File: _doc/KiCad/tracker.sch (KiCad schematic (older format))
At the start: 16 parts

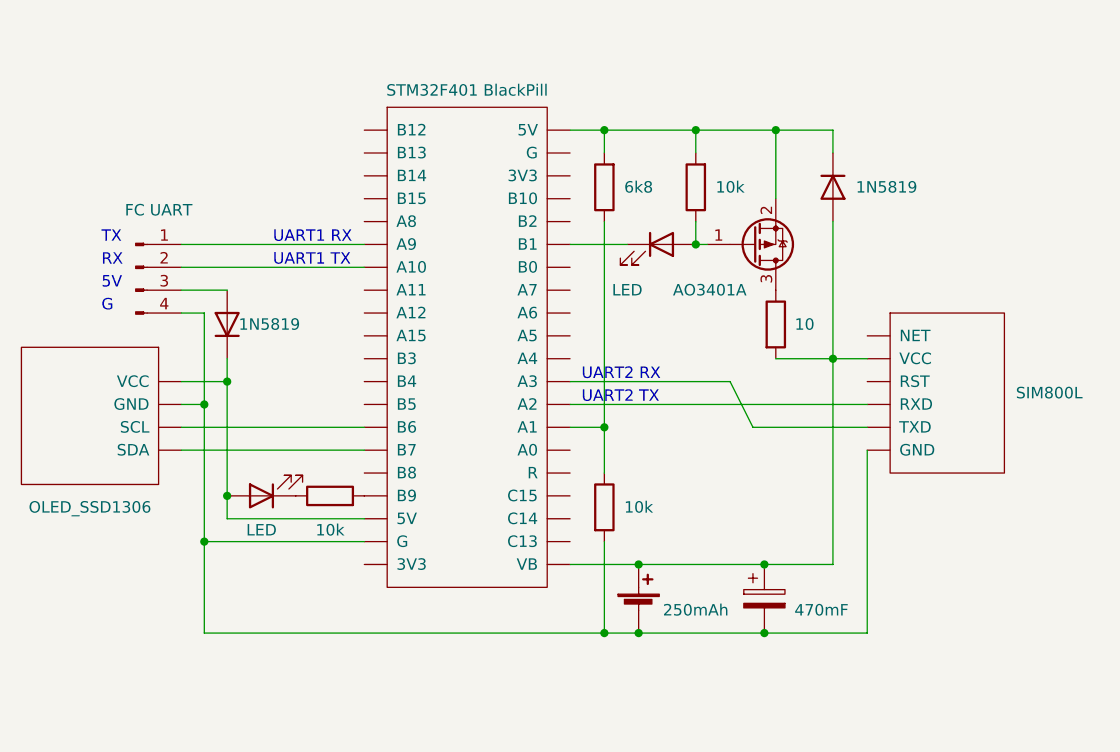
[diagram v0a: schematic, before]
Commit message: Doc: schematic
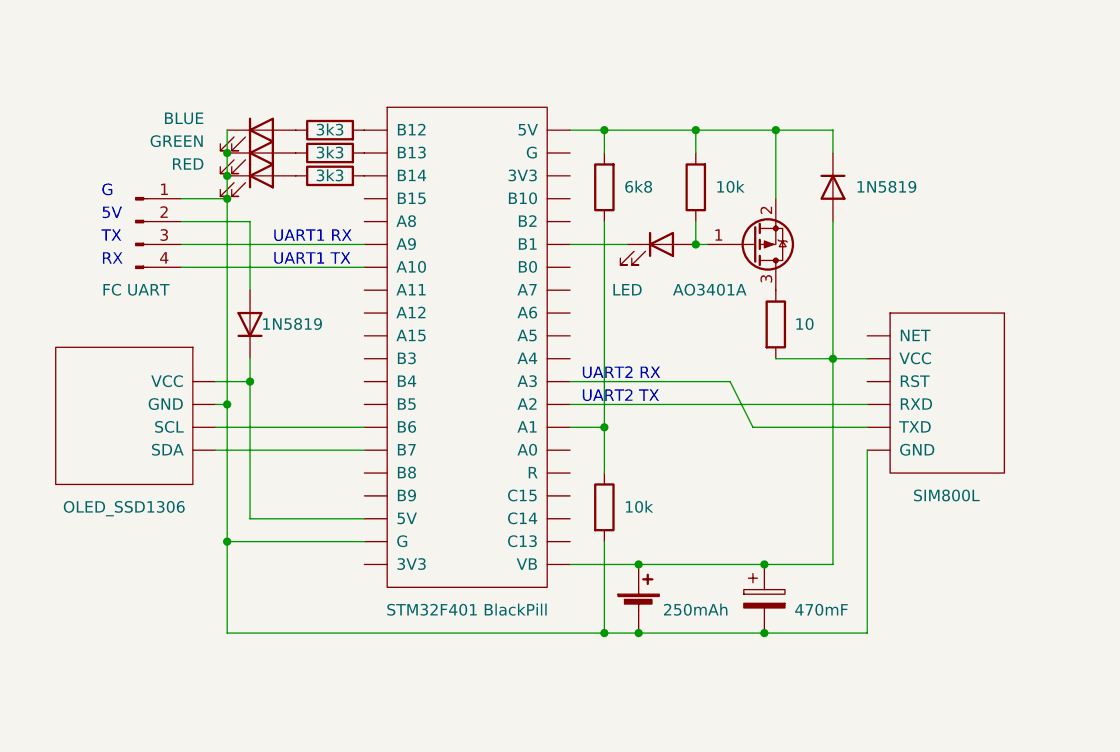
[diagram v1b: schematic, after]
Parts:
- added D?: GREEN, symbol Device:LED
- added D?: RED, symbol Device:LED
- added R? (x2): 3k3, symbol Device:R
- D?: value LED -> BLUE
- R?: value 10k -> 3k3
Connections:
- net at U?.~ (VB): now also R?.2
- net at U?.~ (VCC): no longer U?.~ (VB)
- net at U?.~ (VB), U?.~ (VCC): now also D?.1 (K)
- net at J?.1 (Pin_1), U?.~ (VB): now also BT?.2 (-), C?.2, D?.1 (K), R?.2, U?.~ (VCC), U?.~ (VCC), D?.1 (K), D?.1 (K)
- net at J?.2 (Pin_2): now also D?.2 (A); no longer U?.~ (VB)
- net at J?.3 (Pin_3): now also U?.~ (VB); no longer D?.2 (A)
- net at R?.1: now also D?.2 (A); no longer D?.1 (K)
- new net: U?.~ (VB), U?.~ (VCC) (x4)
- new net: J?.4 (Pin_4), U?.~ (VB)
- new net: R?.2, U?.~ (VB) (x2)
- new net: D?.2 (A), R?.1 (x2)
- now unconnected: U?.~ (VCC), U?.~ (VCC)
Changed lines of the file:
@@
 P 7100 3750
 F 0 "U?" H 7378 3796 50  0001 L CNN
-F 1 "SIM800L" H 7400 3750 50  0000 L CNN
+F 1 "SIM800L" H 6950 3300 50  0000 L CNN
 F 2 "" H 7100 4150 50  0001 C CNN
 F 3 "" H 7100 4150 50  0001 C CNN
@@
 $EndComp
 Wire Wire Line
-	3850 4400 4550 4400
-Wire Wire Line
-	3950 3700 3950 4200
-Wire Wire Line
-	3950 4300 4550 4300
-Wire Wire Line
-	3850 3800 3850 4400
-Connection ~ 3950 3700
-Wire Wire Line
-	3850 3400 3850 3800
-Connection ~ 3850 3800
-Wire Wire Line
-	3850 4400 3850 4800
-Connection ~ 3850 4400
+	3950 4400 4550 4400
+Wire Wire Line
+	4050 4300 4550 4300
+Wire Wire Line
+	3950 3800 3950 4400
+Connection ~ 4050 3700
+Connection ~ 3950 3800
+Wire Wire Line
+	3950 4400 3950 4800
+Connection ~ 3950 4400
 Wire Wire Line
 	5450 3700 6150 3700
 Wire Wire Line
-	3950 3600 3950 3700
+	4050 3600 4050 3700
 $Comp
 L Device:Battery_Cell BT?
@@
 $EndComp
 Wire Wire Line
-	3850 4800 5600 4800
+	3950 4800 5600 4800
 Connection ~ 5750 4500
 Wire Wire Line
@@
 Text Notes 3400 3200 0    50   ~ 0
 RX
-Text Notes 3400 3300 0    50   ~ 0
+Text Notes 3400 3000 0    50   ~ 0
 5V
-Text Notes 3400 3400 0    50   ~ 0
-G
 Connection ~ 6350 2600
 Wire Wire Line
@@
 L Device:D D?
 U 1 1 5FC14E46
-P 3950 3450
-F 0 "D?" V 4050 3400 50  0001 R CNN
-F 1 "1N5819" V 3950 3400 50  0000 R CNN
-F 2 "" H 3950 3450 50  0001 C CNN
-F 3 "~" H 3950 3450 50  0001 C CNN
-	1    3950 3450
+P 4050 3450
+F 0 "D?" V 4150 3400 50  0001 R CNN
+F 1 "1N5819" V 4050 3400 50  0000 R CNN
+F 2 "" H 4050 3450 50  0001 C CNN
+F 3 "~" H 4050 3450 50  0001 C CNN
+	1    4050 3450
 	0    -1   -1   0
 $EndComp
@@
 L myLib:OLED_SSD1306 U?
 U 1 1 5FBCCE2D
-P 3350 3850
-F 0 "U?" H 3350 3500 50  0001 C CNN
-F 1 "OLED_SSD1306" H 3350 3450 50  0000 C CNN
-F 2 "" H 3350 4250 50  0001 C CNN
-F 3 "" H 3350 4250 50  0001 C CNN
-	1    3350 3850
-	1    0    0    -1
-$EndComp
-Wire Wire Line
-	3750 3800 3850 3800
-Wire Wire Line
-	3750 3900 4550 3900
-Wire Wire Line
-	4550 4000 3750 4000
-Wire Wire Line
-	3750 3700 3950 3700
-Wire Wire Line
-	3750 3400 3850 3400
-Wire Wire Line
-	3750 3300 3950 3300
+P 3500 3850
+F 0 "U?" H 3500 3500 50  0001 C CNN
+F 1 "OLED_SSD1306" H 3500 3450 50  0000 C CNN
+F 2 "" H 3500 4250 50  0001 C CNN
+F 3 "" H 3500 4250 50  0001 C CNN
+	1    3500 3850
+	1    0    0    -1
+$EndComp
+Wire Wire Line
+	3900 3800 3950 3800
+Wire Wire Line
+	3900 3900 4550 3900
+Wire Wire Line
+	4550 4000 3900 4000
+Wire Wire Line
+	3900 3700 4050 3700
 Wire Wire Line
 	4550 3200 3750 3200
@@
 L Connector:Conn_01x04_Male J?
 U 1 1 5FBCF7C1
-P 3550 3200
-F 0 "J?" H 3650 3550 50  0001 C CNN
-F 1 "FC UART" H 3650 3450 50  0000 C CNN
-F 2 "" H 3550 3200 50  0001 C CNN
-F 3 "~" H 3550 3200 50  0001 C CNN
-	1    3550 3200
-	1    0    0    -1
-$EndComp
-$Comp
-L Device:R R?
-U 1 1 61E34BAE
-P 4400 4200
-F 0 "R?" H 4250 4150 50  0001 C CNN
-F 1 "10k" V 4250 4200 50  0000 C CNN
-F 2 "" V 4330 4200 50  0001 C CNN
-F 3 "~" H 4400 4200 50  0001 C CNN
-	1    4400 4200
-	0    -1   -1   0
-$EndComp
-$Comp
-L Device:LED D?
-U 1 1 61E372F0
-P 4100 4200
-F 0 "D?" H 3950 4050 50  0001 C CNN
-F 1 "LED" H 4100 4350 50  0000 C CNN
-F 2 "" H 4100 4200 50  0001 C CNN
-F 3 "~" H 4100 4200 50  0001 C CNN
-	1    4100 4200
-	-1   0    0    1
-$EndComp
-Connection ~ 3950 4200
-Wire Wire Line
-	3950 4200 3950 4300
+P 3550 3000
+F 0 "J?" H 3650 3350 50  0001 C CNN
+F 1 "FC UART" H 3550 2700 50  0000 C CNN
+F 2 "" H 3550 3000 50  0001 C CNN
+F 3 "~" H 3550 3000 50  0001 C CNN
+	1    3550 3000
+	1    0    0    -1
+$EndComp
 $Comp
 L myLib:BlackPill U?
@@
 P 5000 3550
 F 0 "U?" H 5000 4765 50  0001 C CNN
-F 1 "STM32F401 BlackPill" H 5000 4674 50  0000 C CNN
+F 1 "STM32F401 BlackPill" H 5000 2400 50  0000 C CNN
 F 2 "" H 5100 4650 50  0001 C CNN
 F 3 "" H 5100 4650 50  0001 C CNN
@@
 	1    0    0    -1
 $EndComp
+Wire Wire Line
+	4050 3700 4050 4300
+Text Notes 3400 2900 0    50   ~ 0
+G
+$Comp
+L Device:R R?
+U 1 1 61E2F3F9
+P 4400 2800
+F 0 "R?" H 4250 2750 50  0001 C CNN
+F 1 "3k3" V 4400 2800 50  0000 C CNN
+F 2 "" V 4330 2800 50  0001 C CNN
+F 3 "~" H 4400 2800 50  0001 C CNN
+	1    4400 2800
+	0    -1   -1   0
+$EndComp
+$Comp
+L Device:R R?
+U 1 1 61E2F33D
+P 4400 2700
+F 0 "R?" H 4250 2650 50  0001 C CNN
+F 1 "3k3" V 4400 2700 50  0000 C CNN
+F 2 "" V 4330 2700 50  0001 C CNN
+F 3 "~" H 4400 2700 50  0001 C CNN
+	1    4400 2700
+	0    -1   -1   0
+$EndComp
+$Comp
+L Device:R R?
+U 1 1 61E34BAE
+P 4400 2600
+F 0 "R?" H 4250 2550 50  0001 C CNN
+F 1 "3k3" V 4400 2600 50  0000 C CNN
+F 2 "" V 4330 2600 50  0001 C CNN
+F 3 "~" H 4400 2600 50  0001 C CNN
+	1    4400 2600
+	0    -1   -1   0
+$EndComp
+$Comp
+L Device:LED D?
+U 1 1 61E2F53B
+P 4100 2800
+F 0 "D?" H 3950 2650 50  0001 C CNN
+F 1 "RED" H 3850 2850 50  0000 R CNN
+F 2 "" H 4100 2800 50  0001 C CNN
+F 3 "~" H 4100 2800 50  0001 C CNN
+	1    4100 2800
+	1    0    0    -1
+$EndComp
+Wire Wire Line
+	3950 2600 3950 2700
+$Comp
+L Device:LED D?
+U 1 1 61E2F4B0
+P 4100 2700
+F 0 "D?" H 3950 2550 50  0001 C CNN
+F 1 "GREEN" H 3850 2750 50  0000 R CNN
+F 2 "" H 4100 2700 50  0001 C CNN
+F 3 "~" H 4100 2700 50  0001 C CNN
+	1    4100 2700
+	1    0    0    -1
+$EndComp
+$Comp
+L Device:LED D?
+U 1 1 61E372F0
+P 4100 2600
+F 0 "D?" H 3950 2450 50  0001 C CNN
+F 1 "BLUE" H 3850 2650 50  0000 R CNN
+F 2 "" H 4100 2600 50  0001 C CNN
+F 3 "~" H 4100 2600 50  0001 C CNN
+	1    4100 2600
+	1    0    0    -1
+$EndComp
+Connection ~ 3950 2700
+Wire Wire Line
+	3950 2700 3950 2800
+Connection ~ 3950 2800
+Wire Wire Line
+	3950 2800 3950 2900
+Wire Wire Line
+	3750 2900 3950 2900
+Connection ~ 3950 2900
+Wire Wire Line
+	3950 2900 3950 3800
+Wire Wire Line
+	3750 3000 4050 3000
+Wire Wire Line
+	4050 3000 4050 3300
 $EndSCHEMATC

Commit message: Doc
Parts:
- removed C?: 470mF, symbol Device:CP
- added C?: 220mF, symbol Device:CP_Small
- added C?: 1000mF, symbol Device:CP_Small
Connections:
- wire segments 50 -> 56
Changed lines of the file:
@@
 Comment4 ""
 $EndDescr
-$Comp
-L myLib:SIM800L U?
-U 1 1 5FBB5448
-P 7100 3750
-F 0 "U?" H 7378 3796 50  0001 L CNN
-F 1 "SIM800L" H 6950 3300 50  0000 L CNN
-F 2 "" H 7100 4150 50  0001 C CNN
-F 3 "" H 7100 4150 50  0001 C CNN
-	1    7100 3750
-	1    0    0    -1
-$EndComp
-Wire Wire Line
-	6150 3700 6250 3900
-Wire Wire Line
-	6750 3600 6600 3600
-$Comp
-L Device:R R?
-U 1 1 5FBC7BFE
-P 5600 2850
-F 0 "R?" H 5450 2800 50  0001 C CNN
-F 1 "6k8" H 5450 2850 50  0000 C CNN
-F 2 "" V 5530 2850 50  0001 C CNN
-F 3 "~" H 5600 2850 50  0001 C CNN
-	1    5600 2850
-	-1   0    0    1
-$EndComp
-$Comp
-L Device:CP C?
-U 1 1 5FBC947C
-P 6300 4650
-F 0 "C?" H 6550 4700 50  0001 C CNN
-F 1 "470mF" H 6550 4600 50  0000 C CNN
-F 2 "" H 6338 4500 50  0001 C CNN
-F 3 "~" H 6300 4650 50  0001 C CNN
-	1    6300 4650
-	1    0    0    -1
-$EndComp
 Wire Wire Line
 	3950 4400 4550 4400
@@
 Connection ~ 3950 4400
 Wire Wire Line
-	5450 3700 6150 3700
-Wire Wire Line
 	4050 3600 4050 3700
-$Comp
-L Device:Battery_Cell BT?
-U 1 1 5FBD92D9
-P 5750 4700
-F 0 "BT?" H 6000 4800 50  0001 C CNN
-F 1 "250mAh" H 6000 4700 50  0000 C CNN
-F 2 "" V 5750 4760 50  0001 C CNN
-F 3 "~" V 5750 4760 50  0001 C CNN
-	1    5750 4700
-	1    0    0    -1
-$EndComp
-Wire Wire Line
-	3950 4800 5600 4800
-Connection ~ 5750 4500
-Wire Wire Line
-	5750 4500 5450 4500
-Connection ~ 5750 4800
-Wire Wire Line
-	5750 4800 6300 4800
-Wire Wire Line
-	6750 4000 6750 4800
-Connection ~ 6300 4500
-Connection ~ 6300 4800
-Wire Wire Line
-	6300 4800 6750 4800
-Wire Wire Line
-	5450 3800 6750 3800
-Wire Wire Line
-	5600 3900 5600 4100
-Wire Wire Line
-	5450 3900 5600 3900
-Wire Wire Line
-	5600 4400 5600 4800
-Connection ~ 5600 4800
-Wire Wire Line
-	5600 4800 5750 4800
-Connection ~ 5600 3900
-Wire Wire Line
-	6750 3900 6250 3900
-Wire Wire Line
-	6350 2600 6350 2900
-Wire Wire Line
-	5450 2600 5600 2600
-$Comp
-L Device:LED D?
-U 1 1 5FC2FAC7
-P 5850 3100
-F 0 "D?" H 5700 2950 50  0001 C CNN
-F 1 "LED" H 5700 2900 50  0000 C CNN
-F 2 "" H 5850 3100 50  0001 C CNN
-F 3 "~" H 5850 3100 50  0001 C CNN
-	1    5850 3100
-	1    0    0    -1
-$EndComp
-Wire Wire Line
-	5450 3100 5700 3100
-Connection ~ 6600 3600
-Wire Wire Line
-	6600 3600 6350 3600
-$Comp
-L Device:R R?
-U 1 1 5FBC87D2
-P 5600 4250
-F 0 "R?" H 5750 4300 50  0001 C CNN
-F 1 "10k" H 5750 4250 50  0000 C CNN
-F 2 "" V 5530 4250 50  0001 C CNN
-F 3 "~" H 5600 4250 50  0001 C CNN
-	1    5600 4250
-	1    0    0    -1
-$EndComp
 Text Notes 4150 3200 0    50   ~ 0
 UART1 TX
 Text Notes 4150 3100 0    50   ~ 0
 UART1 RX\n
-Wire Wire Line
-	5600 2700 5600 2600
-Connection ~ 5600 2600
-Wire Wire Line
-	5600 2600 6000 2600
-Wire Wire Line
-	5600 3000 5600 3900
-Wire Wire Line
-	5750 4500 6300 4500
 Text Notes 3400 3100 0    50   ~ 0
 TX
@@
 Text Notes 3400 3000 0    50   ~ 0
 5V
-Connection ~ 6350 2600
-Wire Wire Line
-	6000 2700 6000 2600
-Connection ~ 6000 2600
-Wire Wire Line
-	6000 2600 6350 2600
-Wire Wire Line
-	6000 3000 6000 3100
-Wire Wire Line
-	6350 2600 6600 2600
-Wire Wire Line
-	6600 3000 6600 3600
-Wire Wire Line
-	6600 2700 6600 2600
-$Comp
-L Device:D D?
-U 1 1 5FC34600
-P 6600 2850
-F 0 "D?" V 6554 2930 50  0001 L CNN
-F 1 "1N5819" V 6600 2950 50  0000 L CNN
-F 2 "" H 6600 2850 50  0001 C CNN
-F 3 "~" H 6600 2850 50  0001 C CNN
-	1    6600 2850
-	0    1    1    0
-$EndComp
-$Comp
-L Device:R R?
-U 1 1 5FC1A3F2
-P 6000 2850
-F 0 "R?" H 5850 2800 50  0001 C CNN
-F 1 "10k" H 5850 2850 50  0000 C CNN
-F 2 "" V 5930 2850 50  0001 C CNN
-F 3 "~" H 6000 2850 50  0001 C CNN
-	1    6000 2850
-	-1   0    0    1
-$EndComp
-$Comp
-L Transistor_FET:AO3401A Q?
-U 1 1 60218619
-P 6250 3100
-F 0 "Q?" H 6000 3250 50  0001 L CNN
-F 1 "AO3401A" H 5900 3300 50  0000 L CNN
-F 2 "Package_TO_SOT_SMD:SOT-23" H 6450 3025 50  0001 L CIN
-F 3 "http://www.aosmd.com/pdfs/datasheet/AO3401A.pdf" H 6250 3100 50  0001 L CNN
-	1    6250 3100
-	1    0    0    1
-$EndComp
-Wire Wire Line
-	6300 4500 6600 4500
-Wire Wire Line
-	6600 4500 6600 3600
-Wire Wire Line
-	6000 3100 6050 3100
-Connection ~ 6000 3100
-Text Notes 5500 3800 0    50   ~ 0
-UART2 TX
-Text Notes 5500 3700 0    50   ~ 0
-UART2 RX\n
 $Comp
 L Device:D D?
@@
 $EndComp
 $Comp
-L Device:R R?
-U 1 1 5FBD5AD0
-P 6350 3450
-F 0 "R?" H 6420 3496 50  0001 L CNN
-F 1 "10" H 6476 3450 50  0000 C CNN
-F 2 "" V 6280 3450 50  0001 C CNN
-F 3 "~" H 6350 3450 50  0001 C CNN
-	1    6350 3450
-	1    0    0    -1
-$EndComp
-$Comp
 L myLib:OLED_SSD1306 U?
 U 1 1 5FBCCE2D
@@
 Wire Wire Line
 	4050 3000 4050 3300
+$Comp
+L myLib:SIM800L U?
+U 1 1 5FBB5448
+P 7350 3750
+F 0 "U?" H 7628 3796 50  0001 L CNN
+F 1 "SIM800L" H 7200 3300 50  0000 L CNN
+F 2 "" H 7350 4150 50  0001 C CNN
+F 3 "" H 7350 4150 50  0001 C CNN
+	1    7350 3750
+	1    0    0    -1
+$EndComp
+Wire Wire Line
+	6400 3700 6500 3900
+Wire Wire Line
+	7000 3600 6850 3600
+Wire Wire Line
+	5450 3700 6400 3700
+Wire Wire Line
+	7000 4000 7000 4800
+Wire Wire Line
+	5450 3800 7000 3800
+Wire Wire Line
+	7000 3900 6500 3900
+Wire Wire Line
+	6600 2600 6600 2900
+$Comp
+L Device:LED D?
+U 1 1 5FC2FAC7
+P 6100 3100
+F 0 "D?" H 5950 2950 50  0001 C CNN
+F 1 "LED" H 5950 2900 50  0000 C CNN
+F 2 "" H 6100 3100 50  0001 C CNN
+F 3 "~" H 6100 3100 50  0001 C CNN
+	1    6100 3100
+	1    0    0    -1
+$EndComp
+Connection ~ 6850 3600
+Wire Wire Line
+	6850 3600 6600 3600
+Connection ~ 6600 2600
+Wire Wire Line
+	6250 2700 6250 2600
+Connection ~ 6250 2600
+Wire Wire Line
+	6250 2600 6600 2600
+Wire Wire Line
+	6250 3000 6250 3100
+Wire Wire Line
+	6600 2600 6850 2600
+Wire Wire Line
+	6850 3000 6850 3600
+Wire Wire Line
+	6850 2700 6850 2600
+$Comp
+L Device:D D?
+U 1 1 5FC34600
+P 6850 2850
+F 0 "D?" V 6804 2930 50  0001 L CNN
+F 1 "1N5819" V 6850 2950 50  0000 L CNN
+F 2 "" H 6850 2850 50  0001 C CNN
+F 3 "~" H 6850 2850 50  0001 C CNN
+	1    6850 2850
+	0    1    1    0
+$EndComp
+$Comp
+L Device:R R?
+U 1 1 5FC1A3F2
+P 6250 2850
+F 0 "R?" H 6100 2800 50  0001 C CNN
+F 1 "10k" H 6100 2850 50  0000 C CNN
+F 2 "" V 6180 2850 50  0001 C CNN
+F 3 "~" H 6250 2850 50  0001 C CNN
+	1    6250 2850
+	-1   0    0    1
+$EndComp
+$Comp
+L Transistor_FET:AO3401A Q?
+U 1 1 60218619
+P 6500 3100
+F 0 "Q?" H 6250 3250 50  0001 L CNN
+F 1 "AO3401A" H 6150 3300 50  0000 L CNN
+F 2 "Package_TO_SOT_SMD:SOT-23" H 6700 3025 50  0001 L CIN
+F 3 "http://www.aosmd.com/pdfs/datasheet/AO3401A.pdf" H 6500 3100 50  0001 L CNN
+	1    6500 3100
+	1    0    0    1
+$EndComp
+Wire Wire Line
+	6850 4500 6850 3600
+Wire Wire Line
+	6250 3100 6300 3100
+Connection ~ 6250 3100
+$Comp
+L Device:R R?
+U 1 1 5FBD5AD0
+P 6600 3450
+F 0 "R?" H 6670 3496 50  0001 L CNN
+F 1 "10" H 6726 3450 50  0000 C CNN
+F 2 "" V 6530 3450 50  0001 C CNN
+F 3 "~" H 6600 3450 50  0001 C CNN
+	1    6600 3450
+	1    0    0    -1
+$EndComp
+Connection ~ 6000 4500
+Connection ~ 6000 4800
+Connection ~ 5850 2600
+Text Notes 5450 3700 0    50   ~ 0
+UART2 RX\n
+Text Notes 5450 3800 0    50   ~ 0
+UART2 TX
+Wire Wire Line
+	5850 3000 5850 3900
+Wire Wire Line
+	5850 2700 5850 2600
+$Comp
+L Device:R R?
+U 1 1 5FBC87D2
+P 5850 4250
+F 0 "R?" H 6000 4300 50  0001 C CNN
+F 1 "10k" H 6000 4250 50  0000 C CNN
+F 2 "" V 5780 4250 50  0001 C CNN
+F 3 "~" H 5850 4250 50  0001 C CNN
+	1    5850 4250
+	1    0    0    -1
+$EndComp
+Wire Wire Line
+	5450 3100 5950 3100
+Connection ~ 5850 3900
+Wire Wire Line
+	5850 4800 6000 4800
+Connection ~ 5850 4800
+Wire Wire Line
+	5850 4400 5850 4800
+Wire Wire Line
+	5450 3900 5850 3900
+Wire Wire Line
+	5850 3900 5850 4100
+Wire Wire Line
+	6000 4500 5450 4500
+$Comp
+L Device:Battery_Cell BT?
+U 1 1 5FBD92D9
+P 6000 4700
+F 0 "BT?" H 6250 4800 50  0001 C CNN
+F 1 "250mAh" H 6250 4700 50  0000 C CNN
+F 2 "" V 6000 4760 50  0001 C CNN
+F 3 "~" V 6000 4760 50  0001 C CNN
+	1    6000 4700
+	1    0    0    -1
+$EndComp
+$Comp
+L Device:R R?
+U 1 1 5FBC7BFE
+P 5850 2850
+F 0 "R?" H 5700 2800 50  0001 C CNN
+F 1 "6k8" H 5700 2850 50  0000 C CNN
+F 2 "" V 5780 2850 50  0001 C CNN
+F 3 "~" H 5850 2850 50  0001 C CNN
+	1    5850 2850
+	-1   0    0    1
+$EndComp
+Wire Wire Line
+	5850 2600 6250 2600
+Wire Wire Line
+	3950 4800 5850 4800
+Wire Wire Line
+	5500 2700 5450 2700
+Wire Wire Line
+	5550 2800 5500 2700
+$Comp
+L Device:CP_Small C?
+U 1 1 63447EEA
+P 5650 2700
+F 0 "C?" H 5738 2746 50  0001 L CNN
+F 1 "220mF" H 5500 2550 50  0000 L CNN
+F 2 "" H 5650 2700 50  0001 C CNN
+F 3 "~" H 5650 2700 50  0001 C CNN
+	1    5650 2700
+	1    0    0    -1
+$EndComp
+Wire Wire Line
+	5450 2600 5650 2600
+Wire Wire Line
+	5650 2800 5550 2800
+Connection ~ 5650 2600
+Wire Wire Line
+	5650 2600 5850 2600
+Wire Wire Line
+	6000 4800 6550 4800
+Wire Wire Line
+	6000 4500 6550 4500
+$Comp
+L Device:CP_Small C?
+U 1 1 6345ADBA
+P 6550 4650
+F 0 "C?" H 6638 4696 50  0001 L CNN
+F 1 "1000mF" H 6650 4600 50  0000 L CNN
+F 2 "" H 6550 4650 50  0001 C CNN
+F 3 "~" H 6550 4650 50  0001 C CNN
+	1    6550 4650
+	1    0    0    -1
+$EndComp
+Wire Wire Line
+	6550 4550 6550 4500
+Connection ~ 6550 4500
+Wire Wire Line
+	6550 4500 6850 4500
+Wire Wire Line
+	6550 4750 6550 4800
+Connection ~ 6550 4800
+Wire Wire Line
+	6550 4800 7000 4800
 $EndSCHEMATC
